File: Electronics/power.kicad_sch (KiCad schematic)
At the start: 44 parts, among them J1 USB_C_Receptacle_USB2.0, Q1 AON3419, Q2 AON3419, SW1 ON_OFF_SWITCH, U2 STUSB4500QTR, U3 BQ25895RTW, U6 NCP186AMX330TAG, U7 MIC2250

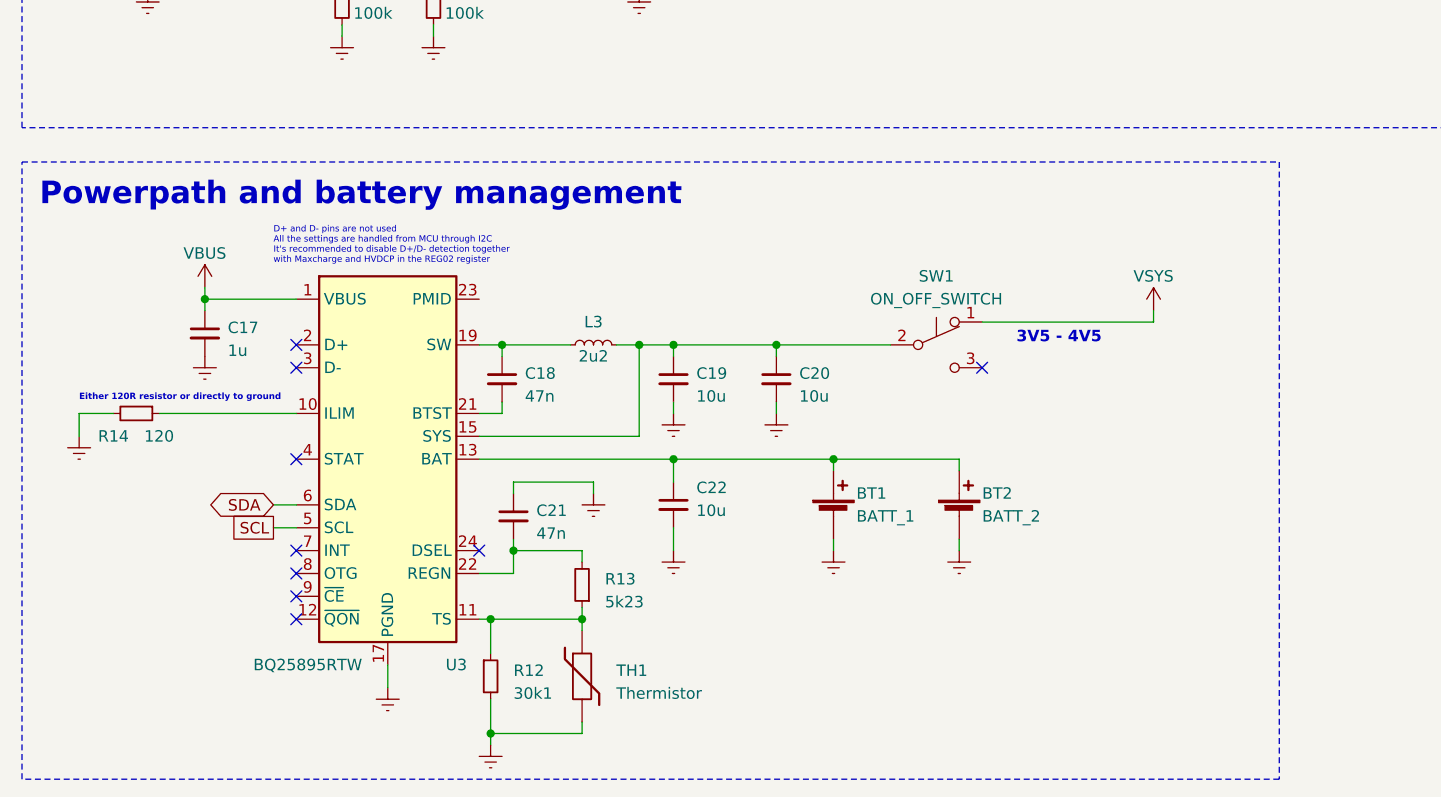
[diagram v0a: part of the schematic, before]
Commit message: All schematics complete
Completed battery, power-path and USB-PD management. 3V3 and V_LIGHTS rail. ESP32-C3 together with Magnetometer, Accelerometer and Gyroscope. And the LED lights
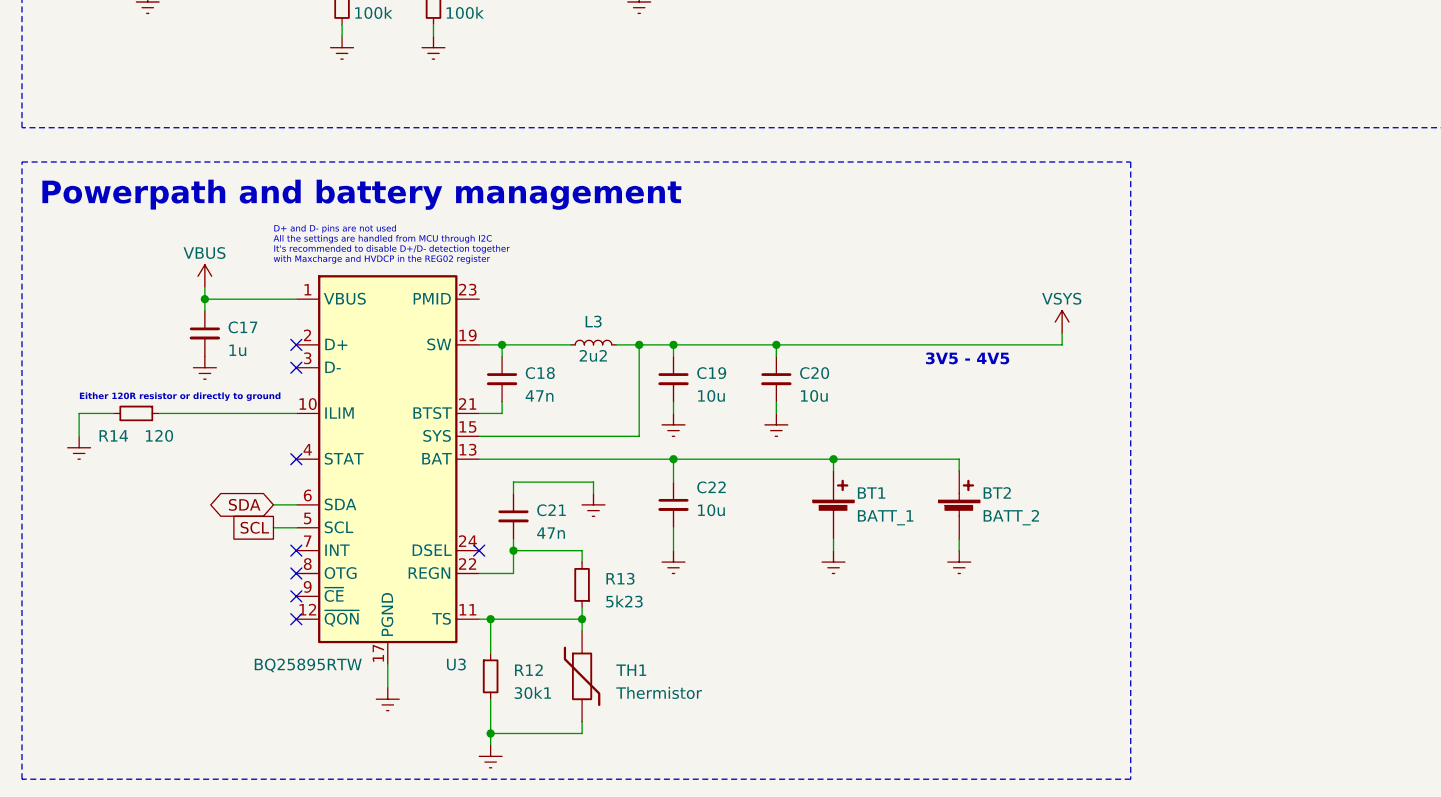
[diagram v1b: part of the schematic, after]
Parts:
- removed SW1: ON_OFF_SWITCH, symbol Switch:SW_Push_SPDT
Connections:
- net VSYS: now also C19.1, C20.1, L3.2, U3.15 (SYS), U3.16 (SYS)
- no-connect marks 18 -> 17
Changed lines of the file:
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@@
   (no_connect (at 48.26 152.4))
   (no_connect (at 46.99 88.9))
-  (no_connect (at 124.46 142.24))
   (no_connect (at 48.26 162.56))
   (wire (pts (xy 201.93 49.53) (xy 201.93 40.64))
@@
     (stroke (width 0) (type default))
   )
-  (wire (pts (xy 124.46 137.16) (xy 143.51 137.16))
-    (stroke (width 0) (type default))
-  )
   (wire (pts (xy 134.62 49.53) (xy 140.97 49.53))
     (stroke (width 0) (type default))
@@
   )
   (wire (pts (xy 80.01 170.18) (xy 80.01 171.45))
+    (stroke (width 0) (type default))
+  )
+  (wire (pts (xy 133.35 139.7) (xy 133.35 138.43))
     (stroke (width 0) (type default))
   )
@@
     (stroke (width 0) (type default))
   )
-  (wire (pts (xy 143.51 137.16) (xy 143.51 135.89))
-    (stroke (width 0) (type default))
-  )
   (wire (pts (xy 201.93 87.63) (xy 204.47 87.63))
     (stroke (width 0) (type default))
@@
     (stroke (width 0) (type default))
   )
-  (wire (pts (xy 101.6 139.7) (xy 114.3 139.7))
+  (wire (pts (xy 101.6 139.7) (xy 133.35 139.7))
     (stroke (width 0) (type default))
   )
@@
   )
   (text_box "Powerpath and battery management"
-    (at 17.78 119.38 0) (size 139.7 68.58)
+    (at 17.78 119.38 0) (size 123.19 68.58)
     (stroke (width 0) (type dash))
     (fill (type none))
@@
     (effects (font (size 0.7 0.7) bold) (justify left bottom))
   )
+  (text "3V5 - 4V5" (at 118.11 142.24 0)
+    (effects (font (size 1.27 1.27) bold) (justify left bottom))
+  )
   (text "Recommended value for R_{1} at 12V output is 240k \nR_{2} value can be calculated as R_{2} = R_{1} / ((V_{OUT} / 1.24) - 1)"
     (at 229.87 30.48 0)
     (effects (font (size 0.75 0.75)) (justify left bottom))
-  )
-  (text "3V5 - 4V5" (at 128.27 139.7 0)
-    (effects (font (size 1.27 1.27) bold) (justify left bottom))
   )
   (text "D+ and D- pins are not used\nAll the settings are handled from MCU through I2C\nIt's recommended to disable D+/D- detection together\nwith Maxcharge and HVDCP in the REG02 register"
@@
         (path "/b70621e2-23d0-406f-b359-5b7c90496935/b637dce6-9faa-48d7-ac20-34c7af1e210c"
           (reference "L4") (unit 1)
-        )
-      )
-    )
-  )
-  (symbol (lib_id "more_power:VSYS") (at 143.51 135.89 0) (unit 1)
-    (in_bom yes) (on_board yes) (dnp no) (fields_autoplaced)
-    (property "Reference" "#PWR043" (at 143.51 139.7 0)
-      (effects (font (size 1.27 1.27)) hide)
-    )
-    (property "Value" "VSYS" (at 143.51 132.08 0)
-      (effects (font (size 1.27 1.27)))
-    )
-    (property "Footprint" "" (at 143.51 135.89 0)
-      (effects (font (size 1.27 1.27)) hide)
-    )
-    (property "Datasheet" "" (at 143.51 135.89 0)
-      (effects (font (size 1.27 1.27)) hide)
-    )
-    (pin "1")
-    (instances
-      (project "Aitken"
-        (path "/b70621e2-23d0-406f-b359-5b7c90496935/b637dce6-9faa-48d7-ac20-34c7af1e210c"
-          (reference "#PWR043") (unit 1)
         )
       )
@@
     )
   )
-  (symbol (lib_id "Switch:SW_Push_SPDT") (at 119.38 139.7 0) (unit 1)
-    (in_bom yes) (on_board yes) (dnp no)
-    (property "Reference" "SW1" (at 119.38 132.08 0)
-      (effects (font (size 1.27 1.27)))
-    )
-    (property "Value" "ON_OFF_SWITCH" (at 119.38 134.62 0)
-      (effects (font (size 1.27 1.27)))
-    )
-    (property "Footprint" "" (at 119.38 139.7 0)
-      (effects (font (size 1.27 1.27)) hide)
-    )
-    (property "Datasheet" "~" (at 119.38 139.7 0)
-      (effects (font (size 1.27 1.27)) hide)
-    )
-    (pin "1")
-    (pin "2")
-    (pin "3")
-    (instances
-      (project "Aitken"
-        (path "/b70621e2-23d0-406f-b359-5b7c90496935/b637dce6-9faa-48d7-ac20-34c7af1e210c"
-          (reference "SW1") (unit 1)
-        )
-      )
-    )
-  )
   (symbol (lib_id "power:Earth") (at 113.03 59.69 0) (unit 1)
     (in_bom yes) (on_board yes) (dnp no) (fields_autoplaced)
@@
         )
       )
+    )
+  )
+  (symbol (lib_id "more_power:VSYS") (at 133.35 138.43 0) (unit 1)
+    (in_bom yes) (on_board yes) (dnp no) (fields_autoplaced)
+    (property "Reference" "#PWR043" (at 133.35 142.24 0)
+      (effects (font (size 1.27 1.27)) hide)
+    )
+    (property "Value" "VSYS" (at 133.35 134.62 0)
+      (effects (font (size 1.27 1.27)))
+    )
+    (property "Footprint" "" (at 133.35 138.43 0)
+      (effects (font (size 1.27 1.27)) hide)
+    )
+    (property "Datasheet" "" (at 133.35 138.43 0)
+      (effects (font (size 1.27 1.27)) hide)
+    )
+    (pin "1")
+    (instances
+      (project "Aitken"
+        (path "/b70621e2-23d0-406f-b359-5b7c90496935/b637dce6-9faa-48d7-ac20-34c7af1e210c"
+          (reference "#PWR043") (unit 1)
+        )
+      )

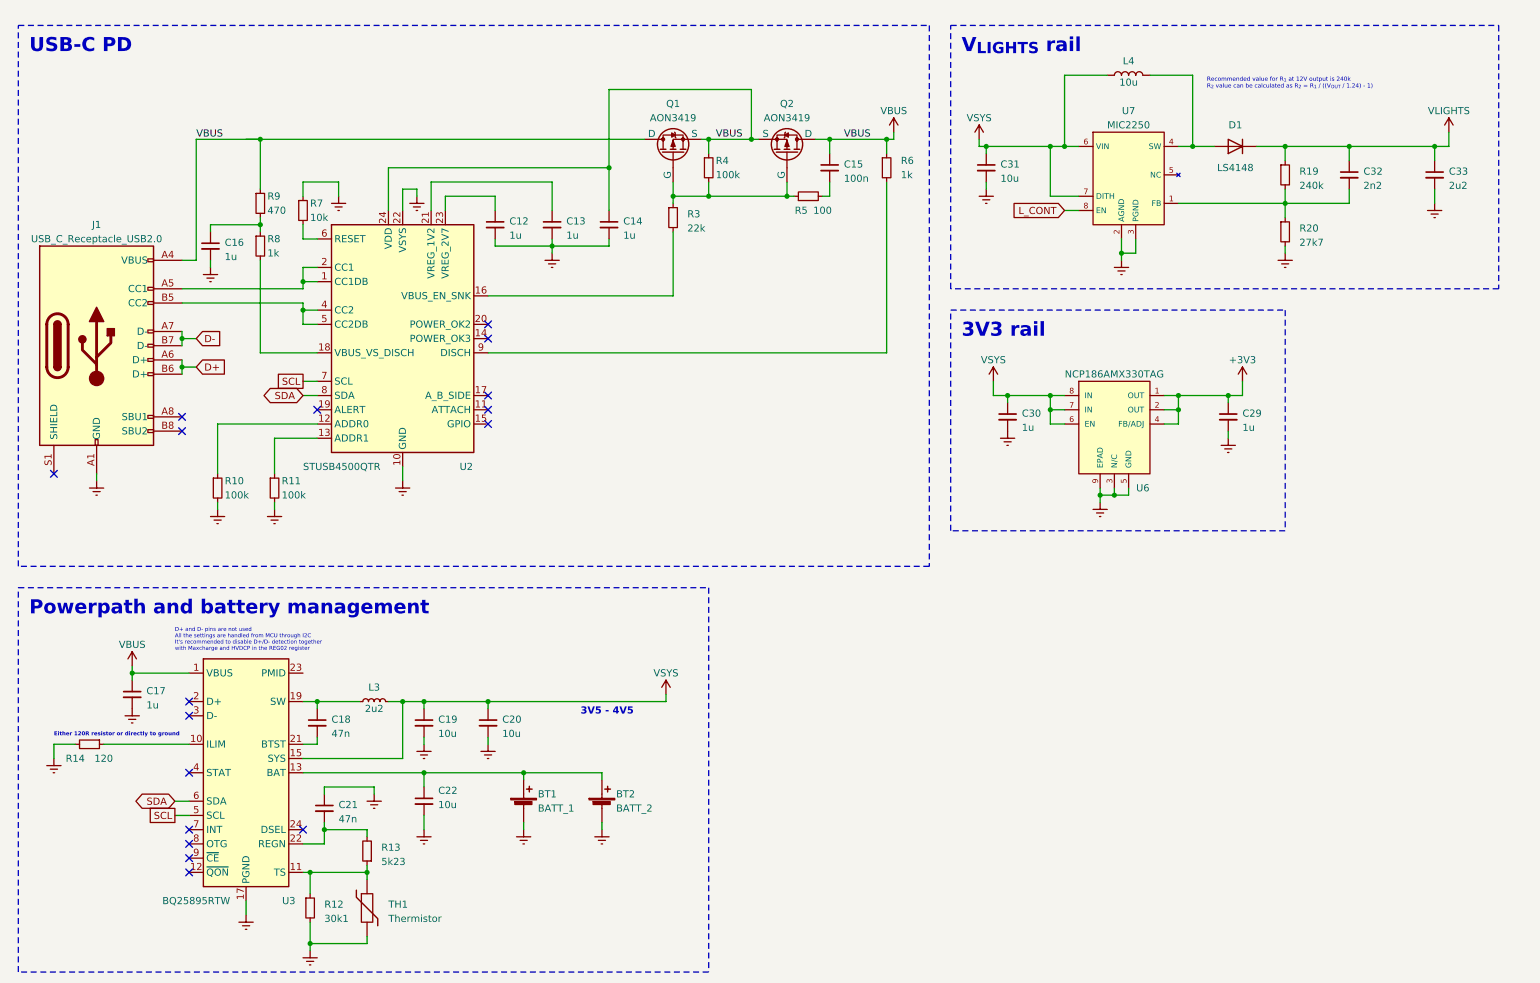
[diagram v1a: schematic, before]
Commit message: Schematic update
Added correct values for crystal capacitors, added net labels and minor cleanup
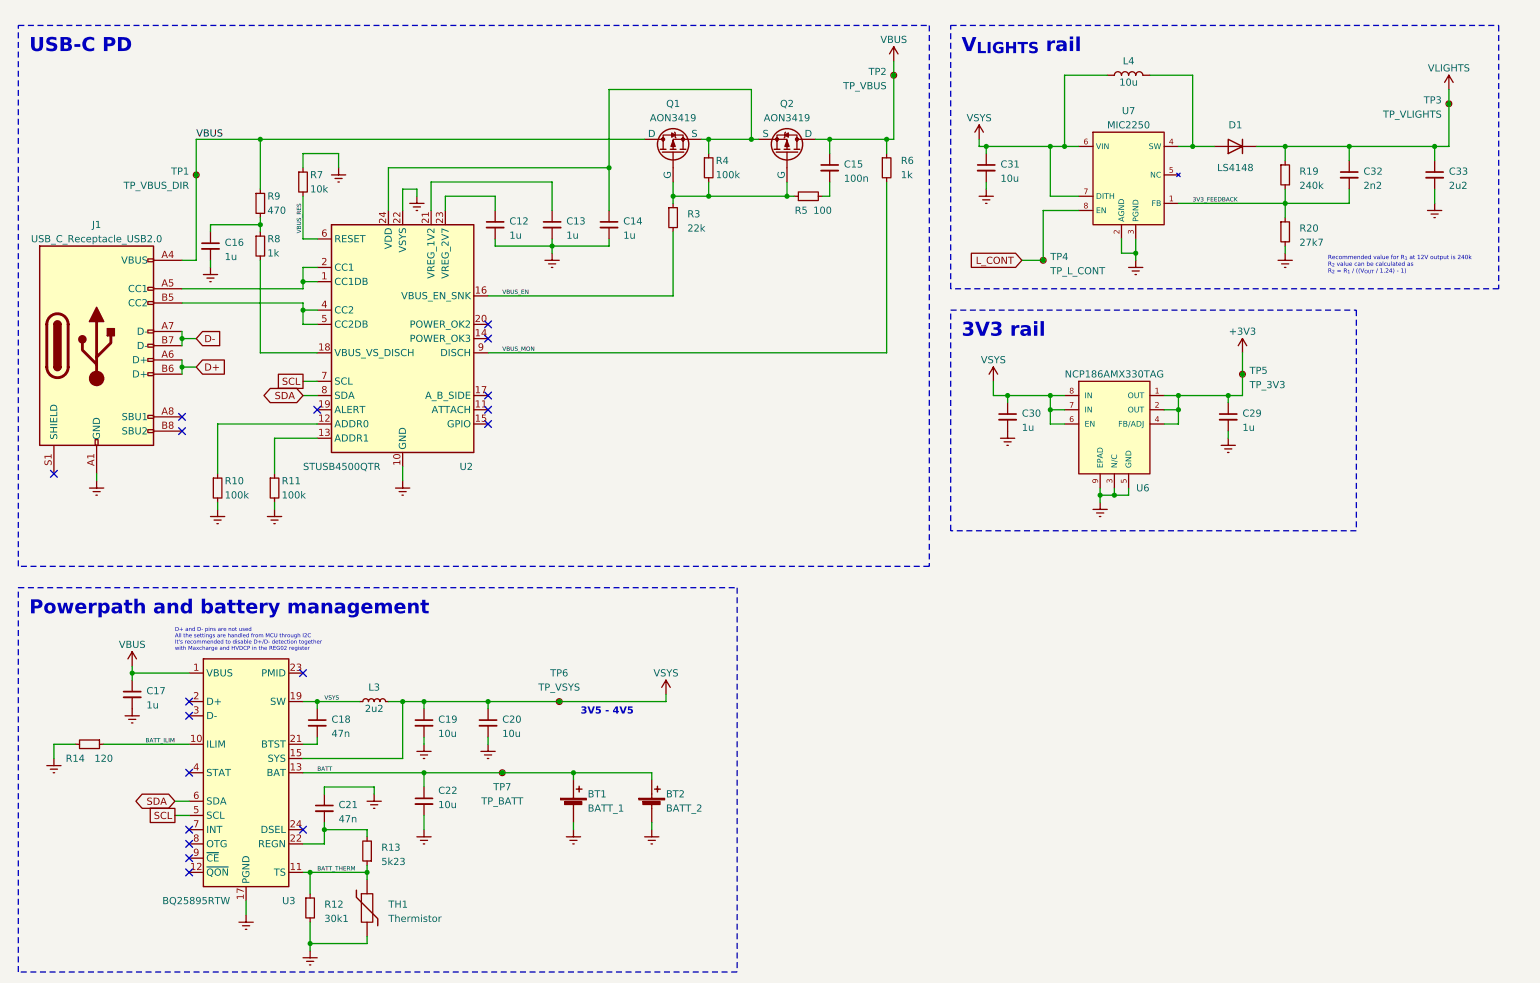
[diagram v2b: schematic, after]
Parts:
- added TP1: TP_VBUS_DIR, symbol Connector:TestPoint_Small
- added TP2: TP_VBUS, symbol Connector:TestPoint_Small
- added TP3: TP_VLIGHTS, symbol Connector:TestPoint_Small
- added TP4: TP_L_CONT, symbol Connector:TestPoint_Small
- added TP5: TP_3V3, symbol Connector:TestPoint_Small
- added TP6: TP_VSYS, symbol Connector:TestPoint_Small
- added TP7: TP_BATT, symbol Connector:TestPoint_Small
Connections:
- net +3V3: now also TP5.1
- net L_CONT: now also TP4.1
- net VBUS: now also TP1.1, TP2.1; no longer C14.1, Q1.3 (S), Q2.3 (S), R4.1, U2.24 (VDD)
- net VLIGHTS: now also TP3.1
- net VSYS: now also C18.1, L3.1, U3.19 (SW), U3.20 (SW), TP6.1
- net BATT: now reaches BT1.1 (+), BT2.1 (+), C22.1, U3.13 (BAT), U3.14 (BAT)
- net BATT: now also TP7.1
- net BATT_THERM: now reaches R12.1, R13.1, TH1.1, U3.11 (TS)
- net 3V3_FEEDBACK: now reaches C32.2, R19.2, R20.1, U7.1 (FB)
- net VBUS_EN: now reaches R3.2, U2.16 (VBUS_EN_SNK)
- net VBUS_RES: now reaches R7.2, U2.6 (RESET)
- net VBUS_MON: now reaches R6.2, U2.9 (DISCH)
- net BATT_ILIM: now reaches R14.1, U3.10 (ILIM)
- new net: C14.1, Q1.3 (S), Q2.3 (S), R4.1, U2.24 (VDD)
- no-connect marks 17 -> 18
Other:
- note removed: "Either 120R resistor or directly to ground"
- moved on the sheet: BT1, BT2, R7
